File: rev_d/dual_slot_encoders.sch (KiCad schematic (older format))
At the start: 16 parts, among them U1 GP1S094HCZ0F, U2 GP1S094HCZ0F, U3 GPS1S97HCZ0F, U4 GPS1S97HCZ0F

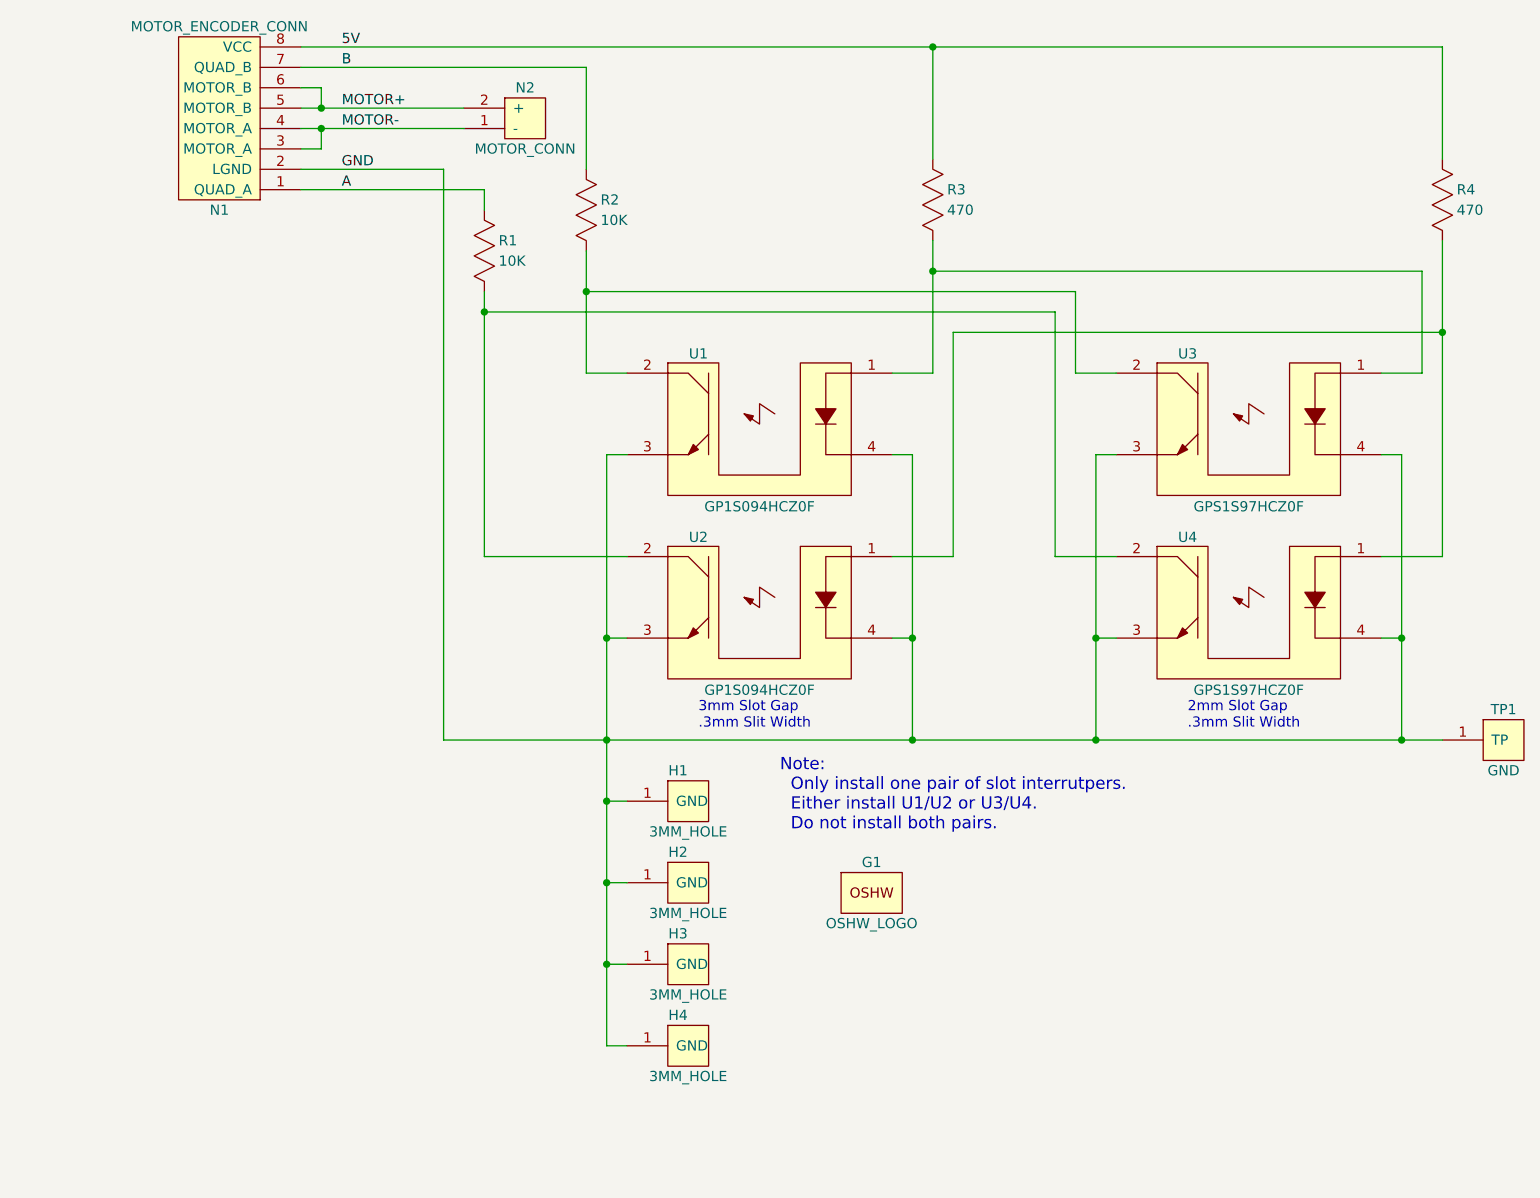
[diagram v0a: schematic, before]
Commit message: Rev. D is pretty much ready.
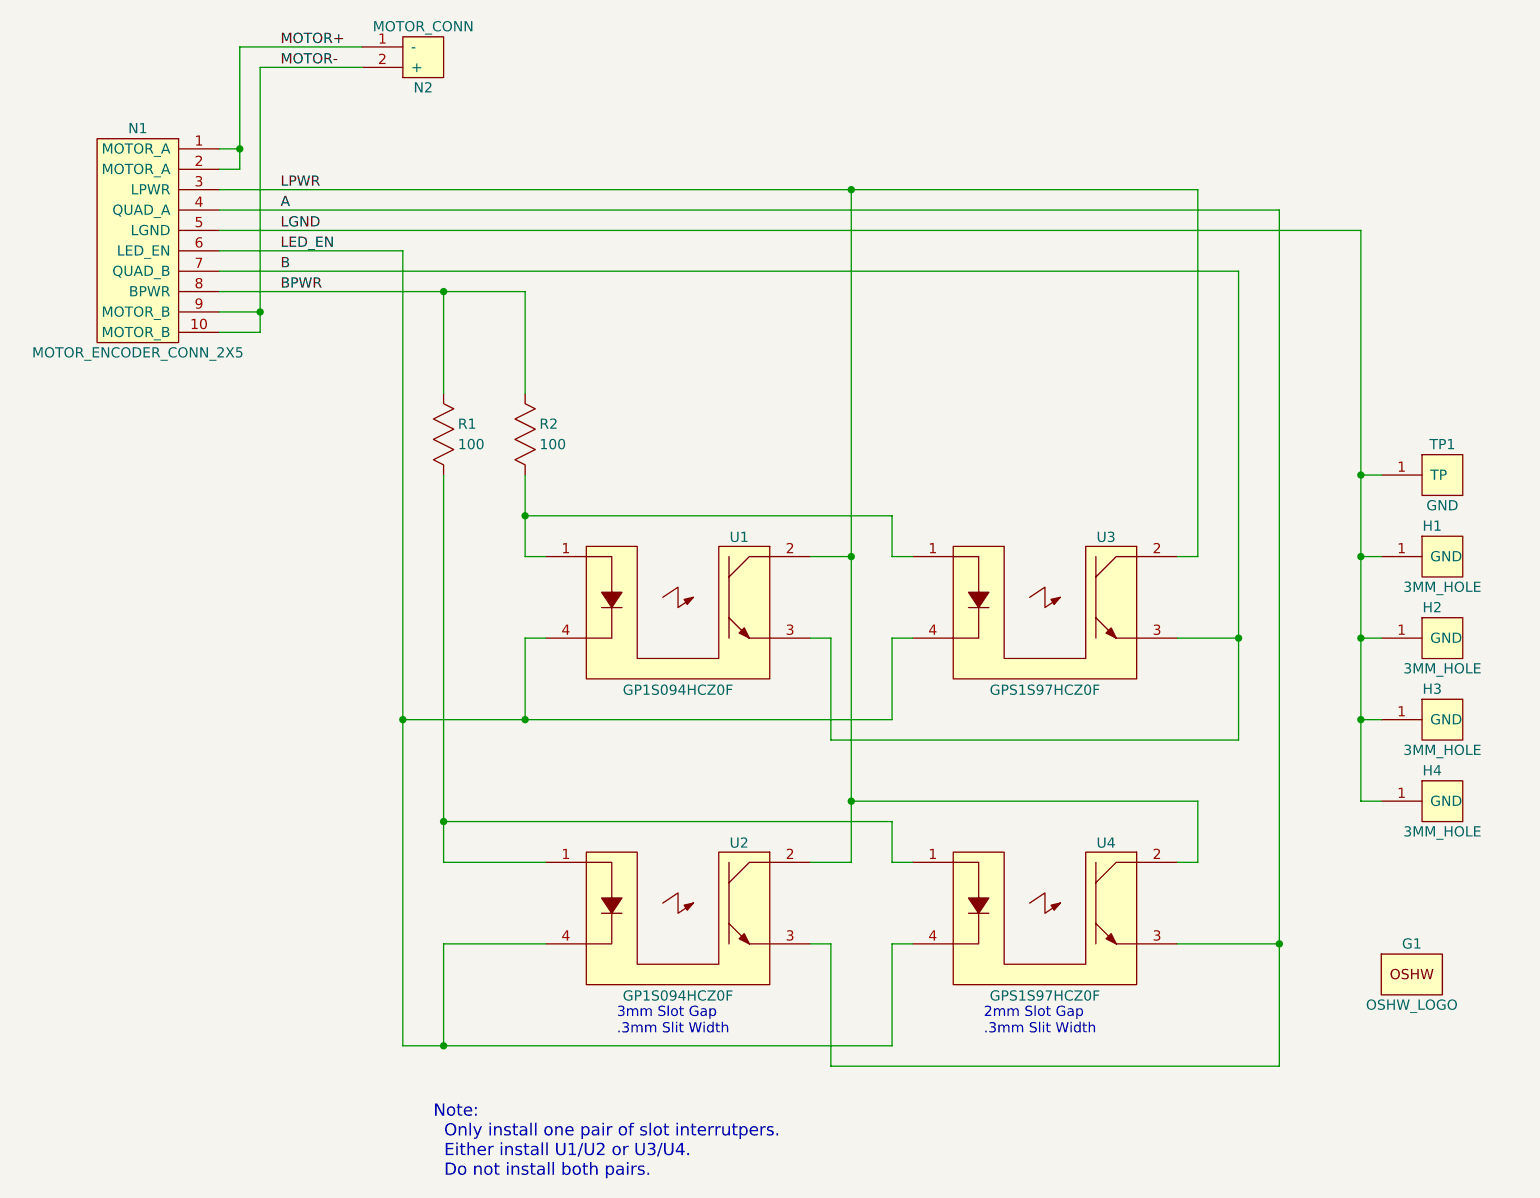
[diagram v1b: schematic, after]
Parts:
- removed N1: MOTOR_ENCODER_CONN, dual_slot_encoders:Pin_Header_Straight_2x04_Shrouded, symbol MOTOR_ENCODER_CONN
- removed R1, R2: 10K, dual_slot_encoders:Resistor_Horizontal_400, symbol R_VERT
- added N1: MOTOR_ENCODER_CONN_2X5, ~, symbol MOTOR_ENCODER_CONN_2X5
- R1: renamed from R4; value 470 -> 100
- R2: renamed from R3; value 470 -> 100
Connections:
- net A: now also U2.3, U4.3, N1.4 (QUAD_A)
- net B: now also U1.3, U3.3, N1.7 (QUAD_B)
- net MOTOR+: now also N2.1 (-), N1.1 (MOTOR_A), N1.2 (MOTOR_A); no longer N2.2 (+)
- net MOTOR-: now also N2.2 (+), N1.10 (MOTOR_B), N1.9 (MOTOR_B); no longer N2.1 (-)
- net LPWR: now reaches U1.2, U3.2
- net LPWR: now also U2.2, U4.2, N1.3 (LPWR)
- net 5V renamed BPWR
- net BPWR: now also N1.8 (BPWR)
- removed net GND: H1.1 (GND), H2.1 (GND), H3.1 (GND), H4.1 (GND), TP1.1 (TP), U1.3, U1.4, U2.3, U2.4, U3.3, U3.4, U4.3, U4.4
- new net LED_EN: N1.6 (LED_EN), U1.4, U2.4, U3.4, U4.4
- new net LGND: H1.1 (GND), H2.1 (GND), H3.1 (GND), H4.1 (GND), N1.5 (LGND), TP1.1 (TP)
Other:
- moved on the sheet: G1, H1, H2, H3, H4, N2, R1, R2, TP1, U1, U2, U3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
